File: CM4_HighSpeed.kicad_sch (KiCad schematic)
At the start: 10 parts, among them J13 1-2199119-5, J15 USB_OTG, J16 Conn_01x02, J3 USB-A-S-VT, J5 690-019-298-412, U11 TPD4EUSB30, U13 RT9742SNGV

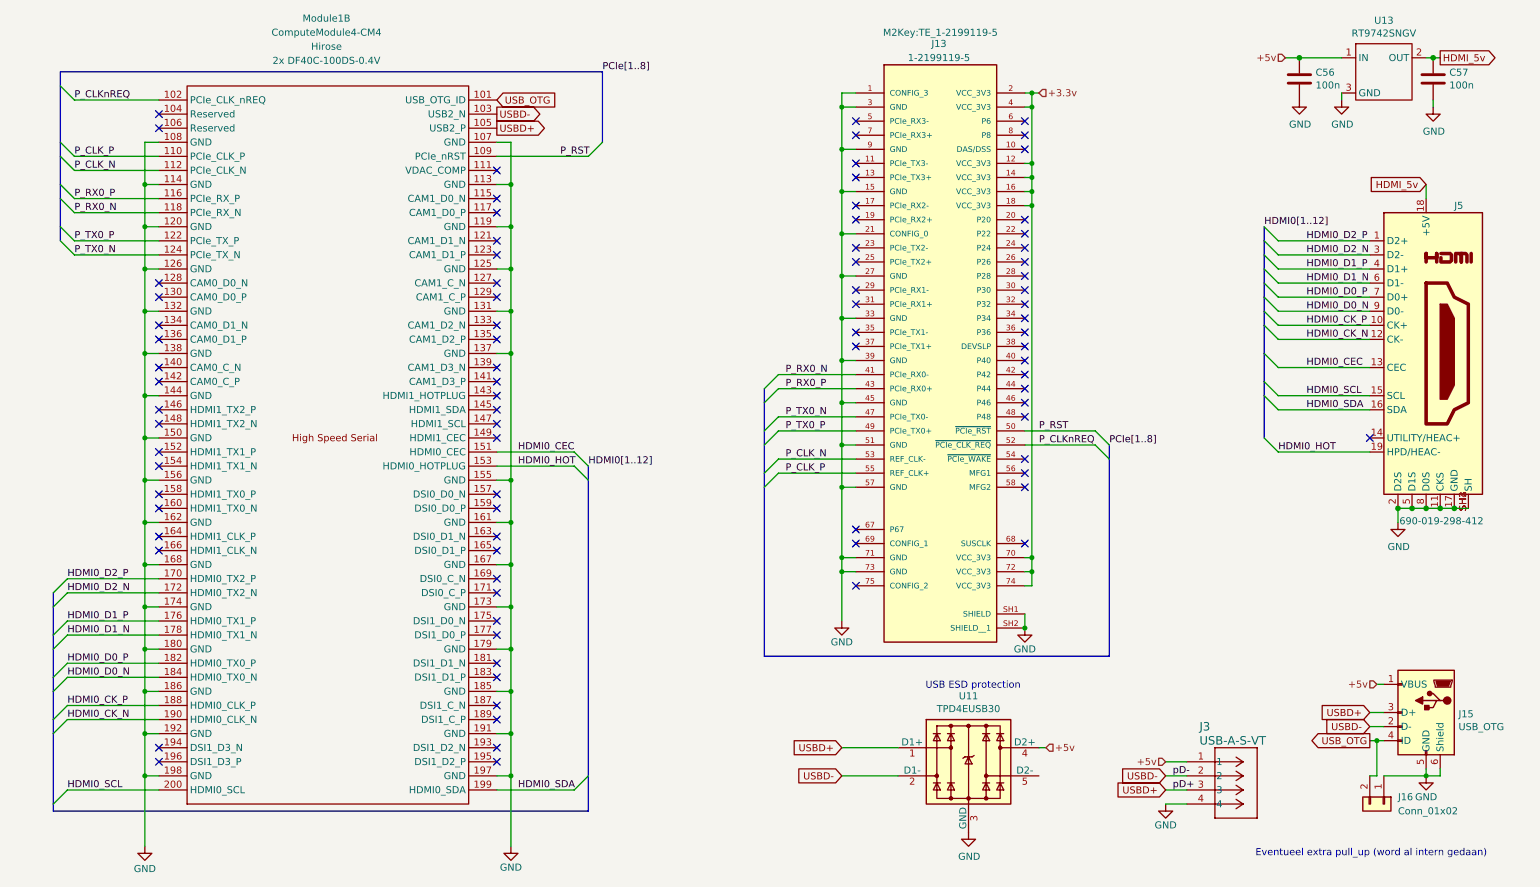
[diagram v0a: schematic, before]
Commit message: Hehe, smol board now
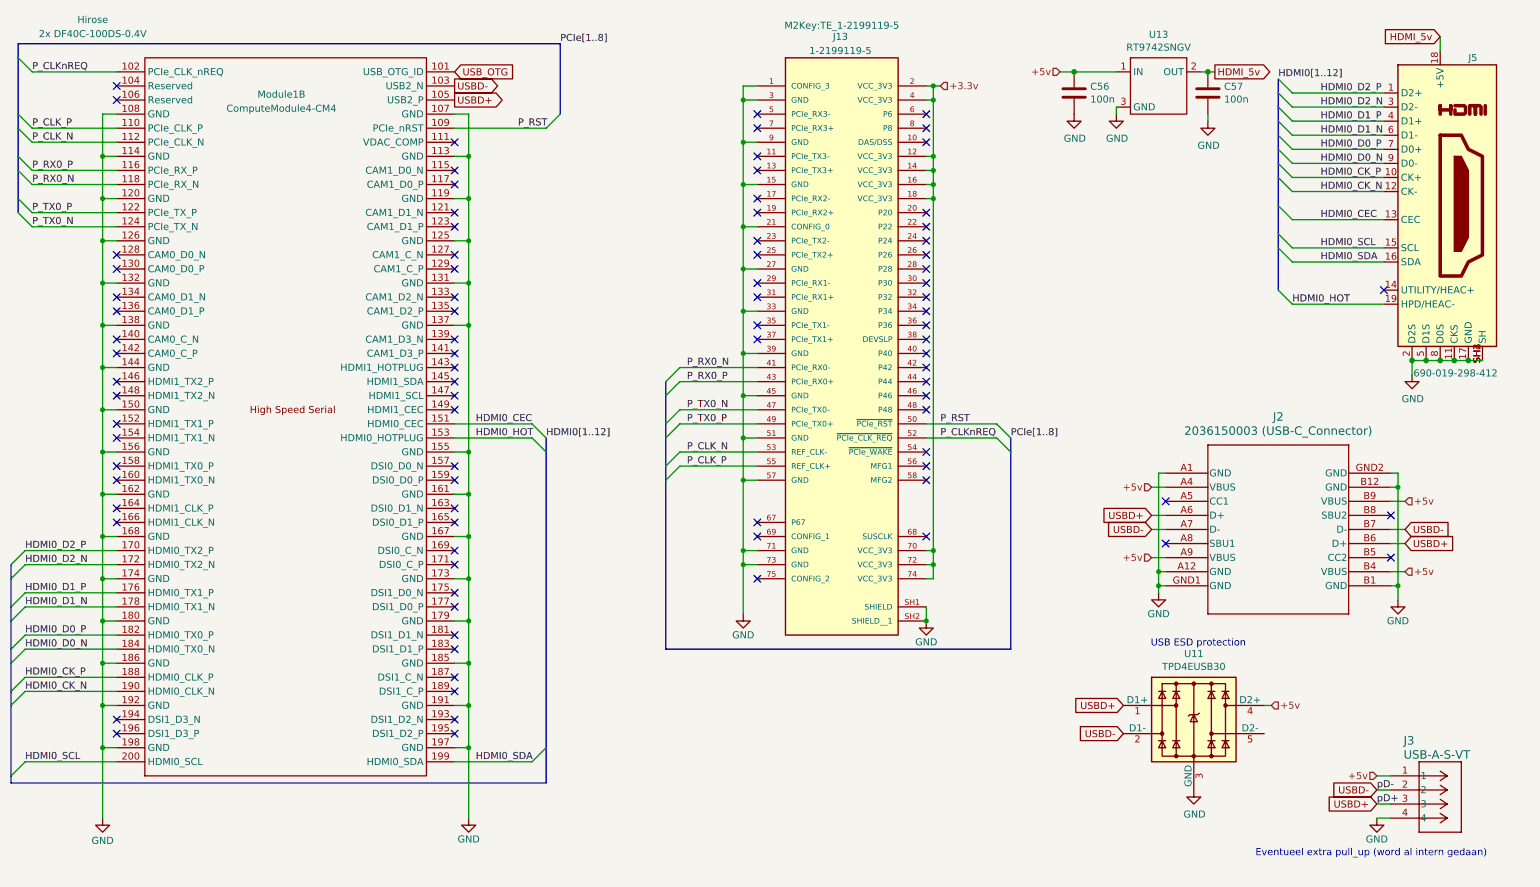
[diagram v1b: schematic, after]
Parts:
- removed J15: USB_OTG, Connector_USB:USB_Micro-B_Amphenol_10103594-0001LF_Horizontal, symbol Connector:USB_OTG
- removed J16: Conn_01x02, Connector_PinHeader_2.54mm:PinHeader_1x02_P2.54mm_Vertical, symbol Connector_Generic:Conn_01x02
- added J2: 2036150003 (USB-C_Connector), USB-C:CONN_2036150003_MOL(USB-c_connector), symbol 2026-03-08_10-34-21:2036150003
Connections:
- net +5v: now also J2.A4 (VBUS), J2.A9 (VBUS), J2.B4 (VBUS), J2.B9 (VBUS)
- net GND: now also J2.A1 (GND), J2.A12 (GND), J2.B1 (GND), J2.B12 (GND), J2.GND1 (GND), J2.GND2 (GND)
- net USBD+: now also J2.A6 (D+), J2.B6 (D+)
- net USBD-: now also J2.A7 (D-), J2.B7 (D-)
- no-connect marks 85 -> 89
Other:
- moved on the sheet: C56, C57, J13, J3, J5, Module1B, U11, U13
